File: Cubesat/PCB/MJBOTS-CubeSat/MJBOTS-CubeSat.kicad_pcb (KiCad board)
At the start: 2 copper layers, 88.1 x 82.7 mm, 23 parts, among them J1 Display, J10 MOTOR3-XT30, J11 JST-BATT, J12 MOTOR3, J2 MPU 6050, J3 Pi_GPIO, J4 CAN, J5 MOTOR1, J6 MOTOR2, J7 INPUT-XT60, J8 MOTOR1-XT30, J9 MOTOR2-XT30, U1 LM2596S, U2 MCP3008-I/SL

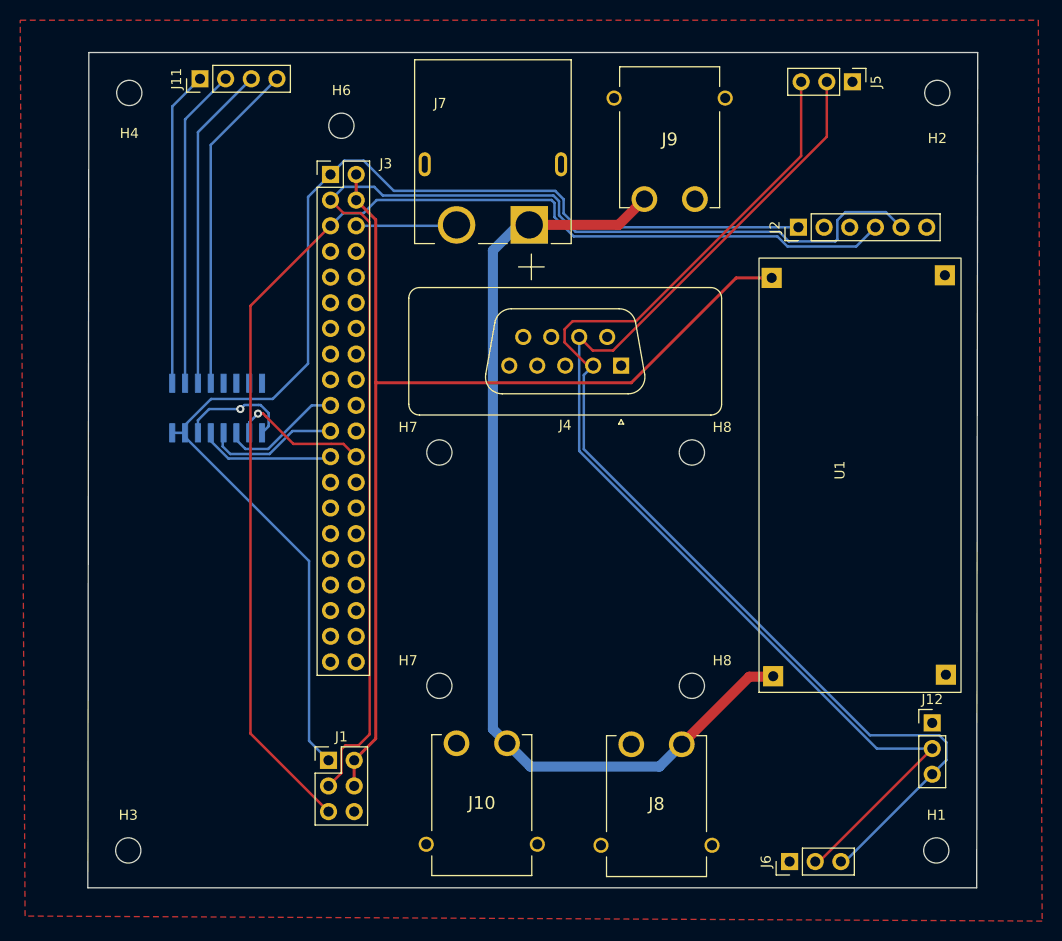
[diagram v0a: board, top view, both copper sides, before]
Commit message: Final Updates "HOPEFULLY"
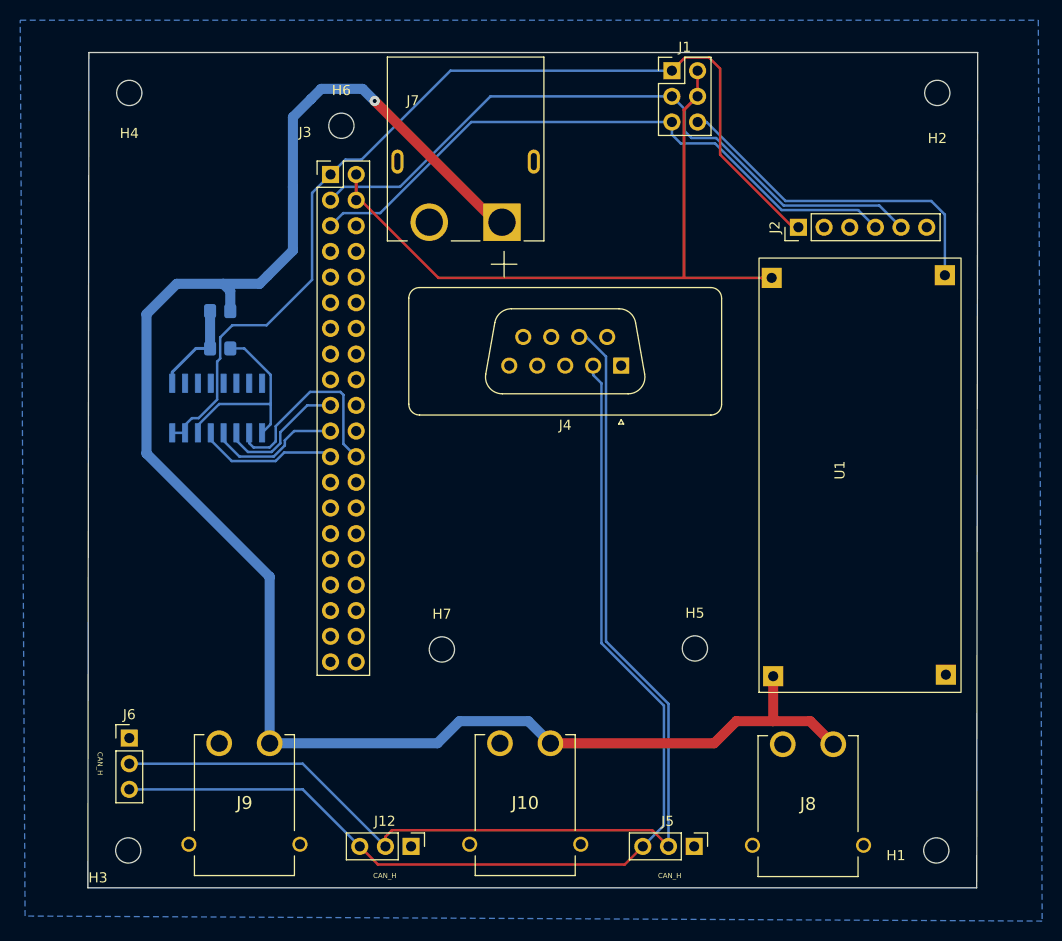
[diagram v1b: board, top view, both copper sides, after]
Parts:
- removed the H7 at (129.7, 84.6)
- removed the H7 at (129.7, 107.7)
- removed H8 (x2): MountingHole, MountingHole:MountingHole_2.5mm
- removed J11: JST-BATT, Connector_PinHeader_2.54mm:PinHeader_1x04_P2.54mm_Vertical
- added H5: MountingHole, MountingHole:MountingHole_2.5mm, F.Cu at (155.0, 104.0)
- added H7: MountingHole, MountingHole:MountingHole_2.5mm, F.Cu at (129.9, 104.1)
- added R1: 2k, Resistor_SMD:R_0805_2012Metric_Pad1.20x1.40mm_HandSolder, B.Cu at (108.0, 70.6)
- added R2: 1k, Resistor_SMD:R_0805_2012Metric_Pad1.20x1.40mm_HandSolder, B.Cu at (108.0, 74.3)
- moved J9 78.0 mm to (110.4, 119.3), turned to 180 degrees
- moved J5 77.3 mm to (154.9, 123.6)
- moved J1 76.3 mm to (152.7, 46.8)
- moved J6 66.5 mm to (99.0, 112.9), turned to 0 degrees
- moved J12 53.0 mm to (126.9, 123.6), turned to -90 degrees
- moved J8 15.0 mm to (166.2, 119.4)
- moved J10 4.30 mm to (138.2, 119.3)
- moved J7 2.71 mm to (132.3, 55.8)
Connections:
- U2 pad 1: /A-D Converter/CELL1 -> /A-D Converter/12V
- U2 pad 2: /A-D Converter/CELL2 -> unconnected-(U2-Pad2)
- U2 pad 3: /A-D Converter/CELL3 -> unconnected-(U2-Pad3)
- U2 pad 4: /A-D Converter/VT -> unconnected-(U2-Pad4)
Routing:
- net /VCC: track 97.5 -> 172.1 mm, vias 0 -> 1
- net /SCL: track 123.0 -> 63.2 mm
- net /SDA: track 126.1 -> 67.4 mm
- net /5V: track 105.7 -> 67.9 mm
- net GND: track 21.4 -> 54.3 mm, vias 1 -> 0
- net /A-D Converter/VT: track 32.9 -> 0.00 mm
- net /A-D Converter/CELL3: track 32.3 -> 0.00 mm
- net /A-D Converter/CELL2: track 31.8 -> 0.00 mm
- net /A-D Converter/CELL1: track 31.3 -> 0.00 mm
- net /3.3V: track 125.1 -> 98.3 mm
- net /CAN_L: track 115.9 -> 106.0 mm
- net /A-D Converter/12V: track 0.00 -> 9.52 mm
- net /CS: track 13.7 -> 20.4 mm, vias 1 -> 0
- net /MOSI: track 12.2 -> 13.1 mm
- net /CAN_H: track 113.9 -> 113.2 mm
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- added copper zone on B.Cu, net GND
- removed copper zone on F.Cu, net GND
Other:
- board text added: "CAN_H"
